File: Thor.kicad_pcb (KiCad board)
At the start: 4 copper layers, 300 x 200 mm, 41 parts, among them J1 Conn_02x32_Counter_Clockwise, J2 Conn_02x32_Counter_Clockwise, J3 Conn_01x01, J4 Conn_01x01, Q1 PHP79NQ08LT, Q2 PHP79NQ08LT, Q3 PHP79NQ08LT, Q4 PHP79NQ08LT, Q5 PHP79NQ08LT, Q6 PHP79NQ08LT, U1 LTC3878

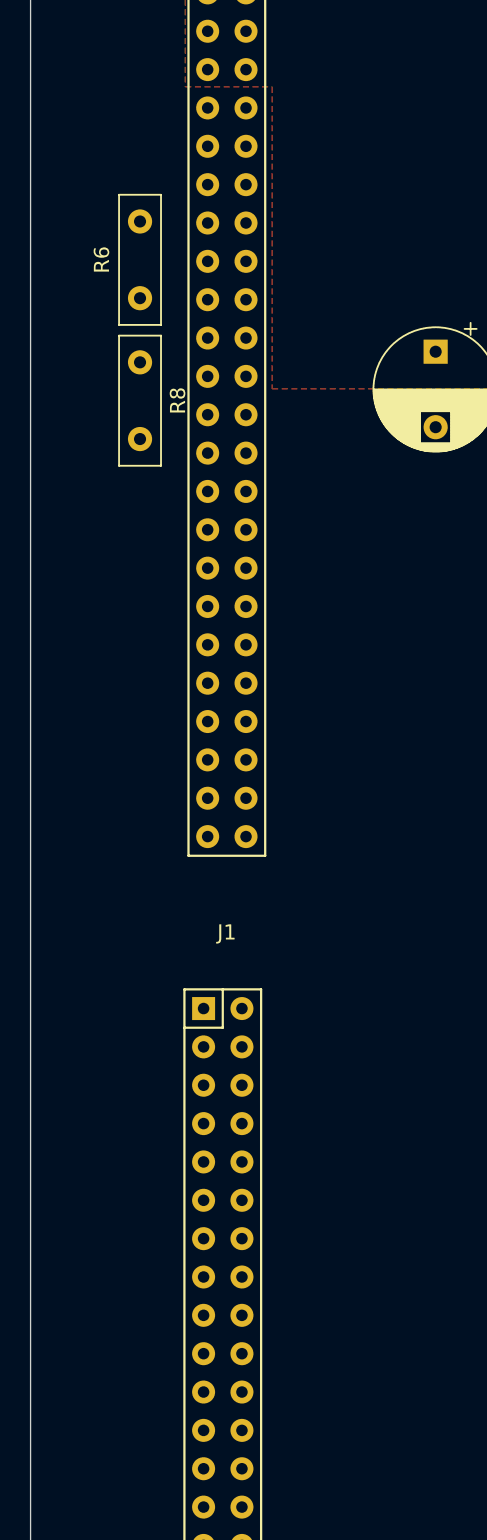
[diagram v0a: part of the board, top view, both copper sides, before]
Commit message: most recent version
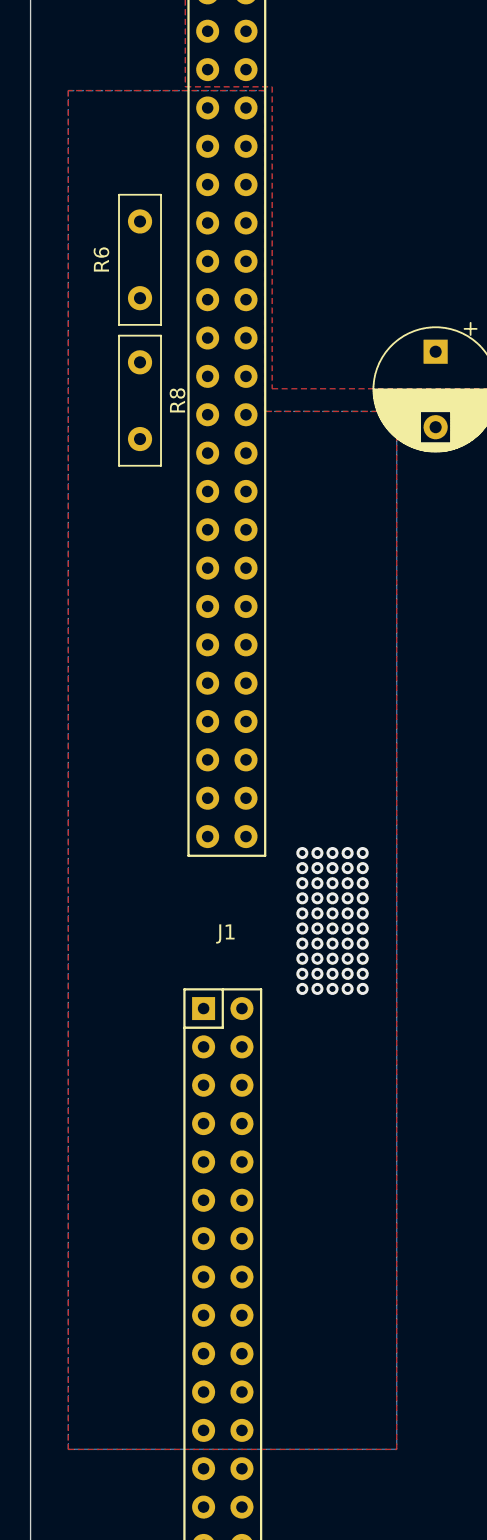
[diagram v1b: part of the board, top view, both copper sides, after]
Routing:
- net /12V_IN: vias 0 -> 50
- added copper zone on B.Cu, net /12V_IN
- added copper zone on F.Cu, net /12V_IN
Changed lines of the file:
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@@
     (thickness 1.6)
     (drawings 4)
-    (tracks 205)
+    (tracks 255)
     (zones 0)
     (modules 41)
@@
   (segment (start 157.9325 88.4) (end 158.48 88.9475) (width 0.25) (layer F.Cu) (net 42))
   (segment (start 156.4875 88.4) (end 157.9325 88.4) (width 0.25) (layer F.Cu) (net 42))
+  (via (at 28 100) (size 0.8) (drill 0.4) (layers F.Cu B.Cu) (net 44))
+  (via (at 29 100) (size 0.8) (drill 0.4) (layers F.Cu B.Cu) (net 44))
+  (via (at 30 100) (size 0.8) (drill 0.4) (layers F.Cu B.Cu) (net 44))
+  (via (at 31 100) (size 0.8) (drill 0.4) (layers F.Cu B.Cu) (net 44))
+  (via (at 32 100) (size 0.8) (drill 0.4) (layers F.Cu B.Cu) (net 44))
+  (via (at 28 101) (size 0.8) (drill 0.4) (layers F.Cu B.Cu) (net 44))
+  (via (at 29 101) (size 0.8) (drill 0.4) (layers F.Cu B.Cu) (net 44))
+  (via (at 30 101) (size 0.8) (drill 0.4) (layers F.Cu B.Cu) (net 44))
+  (via (at 31 101) (size 0.8) (drill 0.4) (layers F.Cu B.Cu) (net 44))
+  (via (at 32 101) (size 0.8) (drill 0.4) (layers F.Cu B.Cu) (net 44))
+  (via (at 28 102) (size 0.8) (drill 0.4) (layers F.Cu B.Cu) (net 44))
+  (via (at 29 102) (size 0.8) (drill 0.4) (layers F.Cu B.Cu) (net 44))
+  (via (at 30 102) (size 0.8) (drill 0.4) (layers F.Cu B.Cu) (net 44))
+  (via (at 31 102) (size 0.8) (drill 0.4) (layers F.Cu B.Cu) (net 44))
+  (via (at 32 102) (size 0.8) (drill 0.4) (layers F.Cu B.Cu) (net 44))
+  (via (at 28 103) (size 0.8) (drill 0.4) (layers F.Cu B.Cu) (net 44))
+  (via (at 29 103) (size 0.8) (drill 0.4) (layers F.Cu B.Cu) (net 44))
+  (via (at 30 103) (size 0.8) (drill 0.4) (layers F.Cu B.Cu) (net 44))
+  (via (at 31 103) (size 0.8) (drill 0.4) (layers F.Cu B.Cu) (net 44))
+  (via (at 32 103) (size 0.8) (drill 0.4) (layers F.Cu B.Cu) (net 44))
+  (via (at 28 104) (size 0.8) (drill 0.4) (layers F.Cu B.Cu) (net 44))
+  (via (at 29 104) (size 0.8) (drill 0.4) (layers F.Cu B.Cu) (net 44))
+  (via (at 30 104) (size 0.8) (drill 0.4) (layers F.Cu B.Cu) (net 44))
+  (via (at 31 104) (size 0.8) (drill 0.4) (layers F.Cu B.Cu) (net 44))
+  (via (at 32 104) (size 0.8) (drill 0.4) (layers F.Cu B.Cu) (net 44))
+  (via (at 28 105) (size 0.8) (drill 0.4) (layers F.Cu B.Cu) (net 44))
+  (via (at 29 105) (size 0.8) (drill 0.4) (layers F.Cu B.Cu) (net 44))
+  (via (at 30 105) (size 0.8) (drill 0.4) (layers F.Cu B.Cu) (net 44))
+  (via (at 31 105) (size 0.8) (drill 0.4) (layers F.Cu B.Cu) (net 44))
+  (via (at 32 105) (size 0.8) (drill 0.4) (layers F.Cu B.Cu) (net 44))
+  (via (at 28 106) (size 0.8) (drill 0.4) (layers F.Cu B.Cu) (net 44))
+  (via (at 29 106) (size 0.8) (drill 0.4) (layers F.Cu B.Cu) (net 44))
+  (via (at 30 106) (size 0.8) (drill 0.4) (layers F.Cu B.Cu) (net 44))
+  (via (at 31 106) (size 0.8) (drill 0.4) (layers F.Cu B.Cu) (net 44))
+  (via (at 32 106) (size 0.8) (drill 0.4) (layers F.Cu B.Cu) (net 44))
+  (via (at 28 107) (size 0.8) (drill 0.4) (layers F.Cu B.Cu) (net 44))
+  (via (at 29 107) (size 0.8) (drill 0.4) (layers F.Cu B.Cu) (net 44))
+  (via (at 30 107) (size 0.8) (drill 0.4) (layers F.Cu B.Cu) (net 44))
+  (via (at 31 107) (size 0.8) (drill 0.4) (layers F.Cu B.Cu) (net 44))
+  (via (at 32 107) (size 0.8) (drill 0.4) (layers F.Cu B.Cu) (net 44))
+  (via (at 28 108) (size 0.8) (drill 0.4) (layers F.Cu B.Cu) (net 44))
+  (via (at 29 108) (size 0.8) (drill 0.4) (layers F.Cu B.Cu) (net 44))
+  (via (at 30 108) (size 0.8) (drill 0.4) (layers F.Cu B.Cu) (net 44))
+  (via (at 31 108) (size 0.8) (drill 0.4) (layers F.Cu B.Cu) (net 44))
+  (via (at 32 108) (size 0.8) (drill 0.4) (layers F.Cu B.Cu) (net 44))
+  (via (at 28 109) (size 0.8) (drill 0.4) (layers F.Cu B.Cu) (net 44))
+  (via (at 29 109) (size 0.8) (drill 0.4) (layers F.Cu B.Cu) (net 44))
+  (via (at 30 109) (size 0.8) (drill 0.4) (layers F.Cu B.Cu) (net 44))
+  (via (at 31 109) (size 0.8) (drill 0.4) (layers F.Cu B.Cu) (net 44))
+  (via (at 32 109) (size 0.8) (drill 0.4) (layers F.Cu B.Cu) (net 44))
   (zone (net 32) (net_name /SW) (layer F.Cu) (hatch edge 0.508)
     (connect_pads yes (clearance 0.508))
@@
       )
     )
+  )
+  (zone (net 44) (net_name /12V_IN) (layer F.Cu) (hatch edge 0.508)
+    (connect_pads yes (clearance 0.508))
+    (min_thickness 0.254)
+    (fill yes (arc_segments 32) (thermal_gap 0.508) (thermal_bridge_width 5))
+    (polygon
+      (pts
+        (xy 25.5 49.5) (xy 12.5 49.5) (xy 12.5 139.5) (xy 34.25 139.5) (xy 34.25 70.75)
+        (xy 25.5 70.75)
+      )
+    )
+  )
+  (zone (net 44) (net_name /12V_IN) (layer B.Cu) (hatch edge 0.508)
+    (connect_pads yes (clearance 0.508))
+    (min_thickness 0.254)
+    (fill yes (arc_segments 32) (thermal_gap 0.508) (thermal_bridge_width 5))
+    (polygon
+      (pts
+        (xy 12.5 49.5) (xy 25.5 49.5) (xy 25.5 70.75) (xy 34.25 70.75) (xy 34.25 139.5)
+        (xy 12.5 139.5)
+      )
+    )
